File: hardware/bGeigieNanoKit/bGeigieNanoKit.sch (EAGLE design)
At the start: 34 parts, among them T1 2SC1815

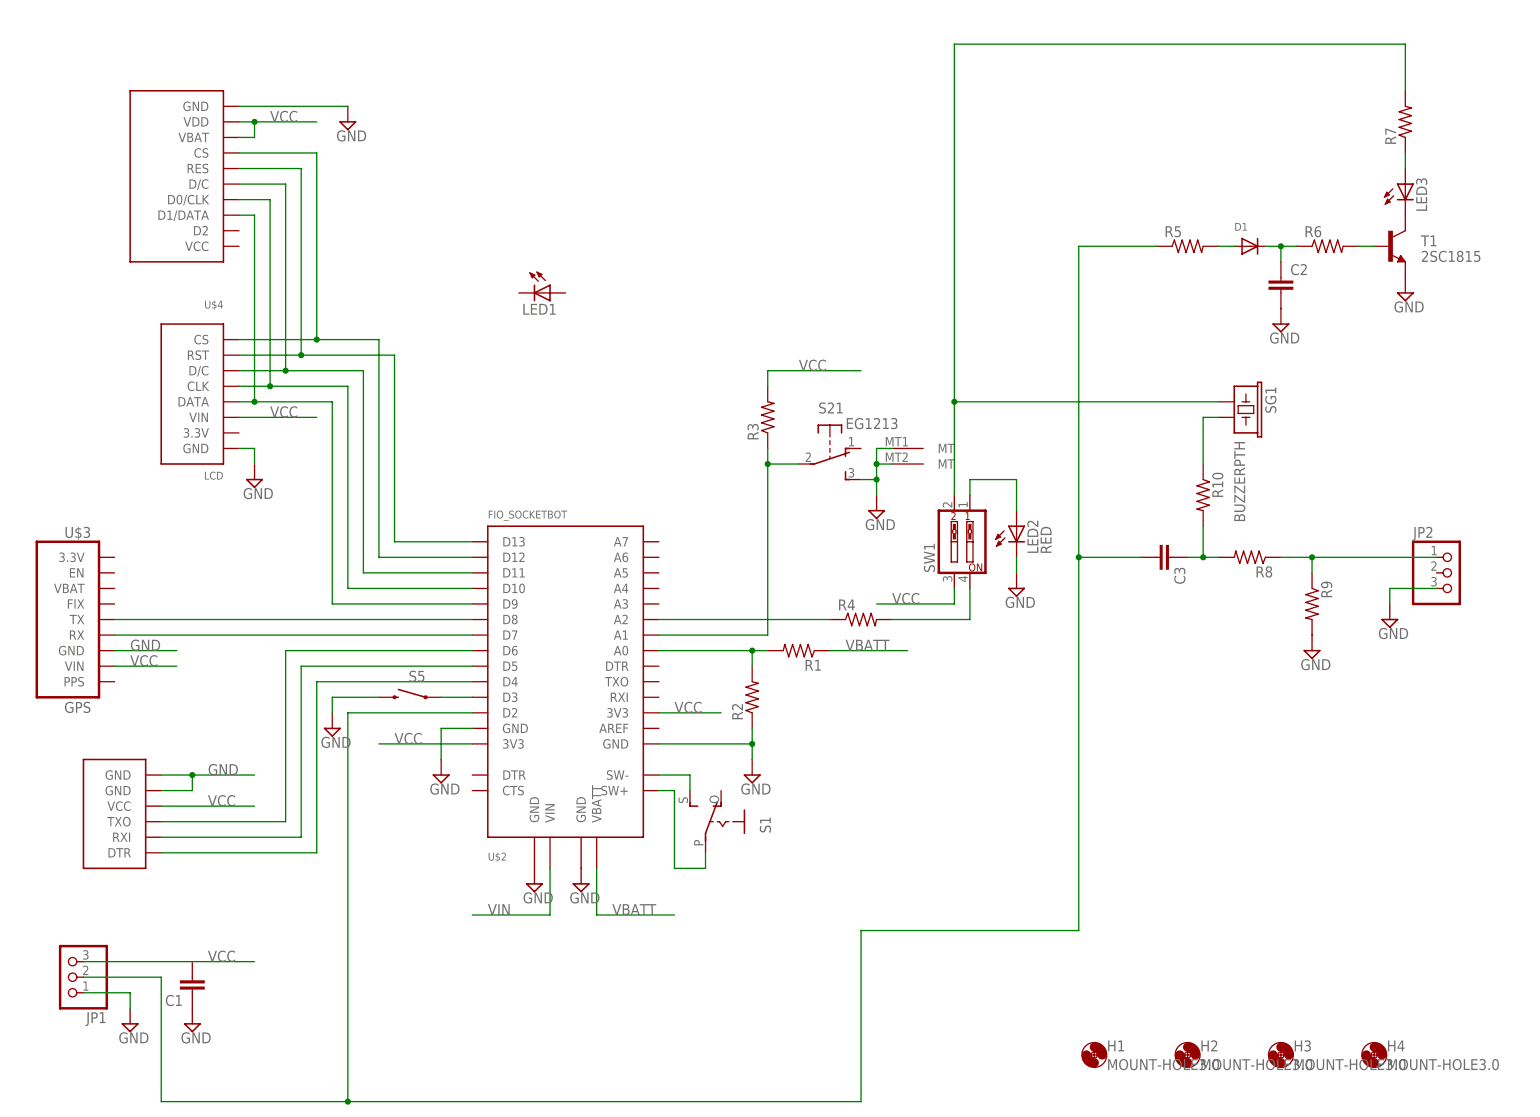
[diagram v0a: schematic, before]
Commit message: fully routed board
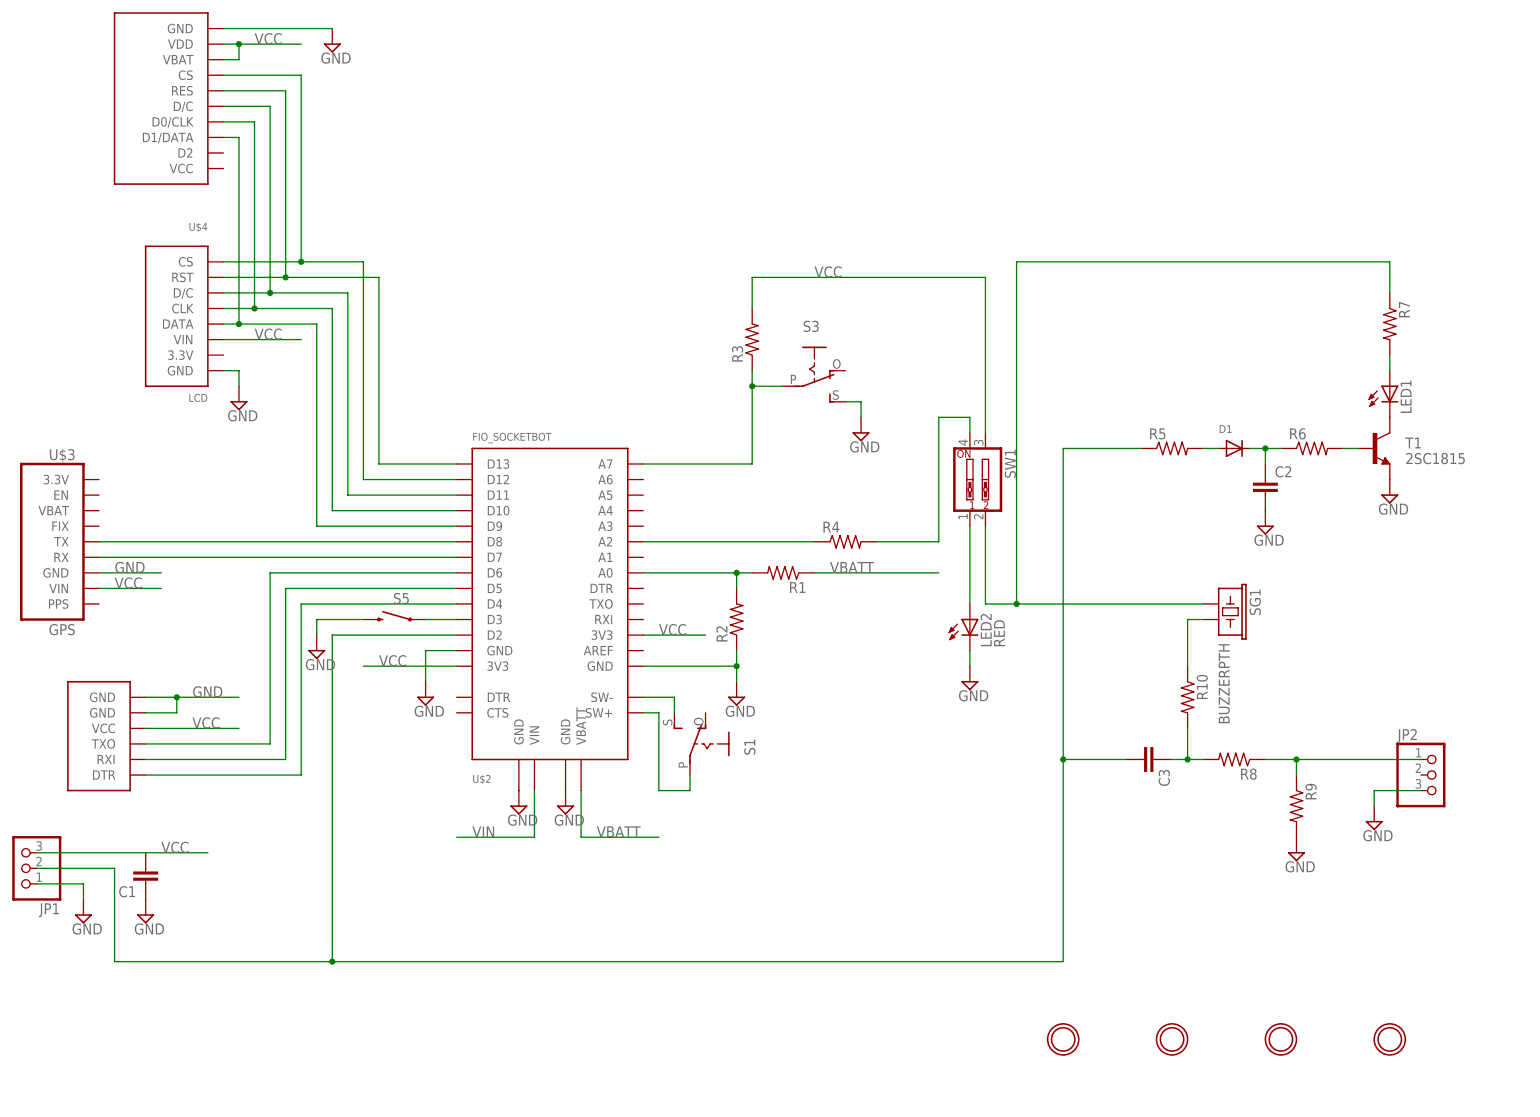
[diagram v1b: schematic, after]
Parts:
- removed H1, H2, H3, H4: MOUNT-HOLE3.0, holes:MOUNT-HOLE3.0
- removed LED3: (no value), adafruit:LED3MM
- removed S2: EG1213, adafruit:EG1213
- added S3: (no value), adafruit:EG1218S
- added U$6, U$7, U$8, U$9: MOUNTINGHOLE3.0THIN, microbuilder:MOUNTINGHOLE3.0THIN
- SW1: device SparkFun:SW_DIP-2 -> special:SW_DIP-2
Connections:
- net GND: now also S3.S; no longer S21.S, S2G$1.MT, S2G$2.MT
- net N$14: now also S3.P, U$2.A7; no longer S21.P, U$2.A1
- net N$19: now also LED1.A, R7.2; no longer LED3.A, R7.1
- net N$21: now also R7.1; no longer R7.2
- net N$22: now also LED1.C; no longer LED3.C
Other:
- moved on the sheet: C1, C2, C3, D1, JP1, JP2, LED1, LED2, R1, R10, R2, R3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
